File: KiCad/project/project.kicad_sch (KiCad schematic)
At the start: 27 parts, among them P1 TerminalBlock 5P 5.0mm, U1 DRV8313PWPR

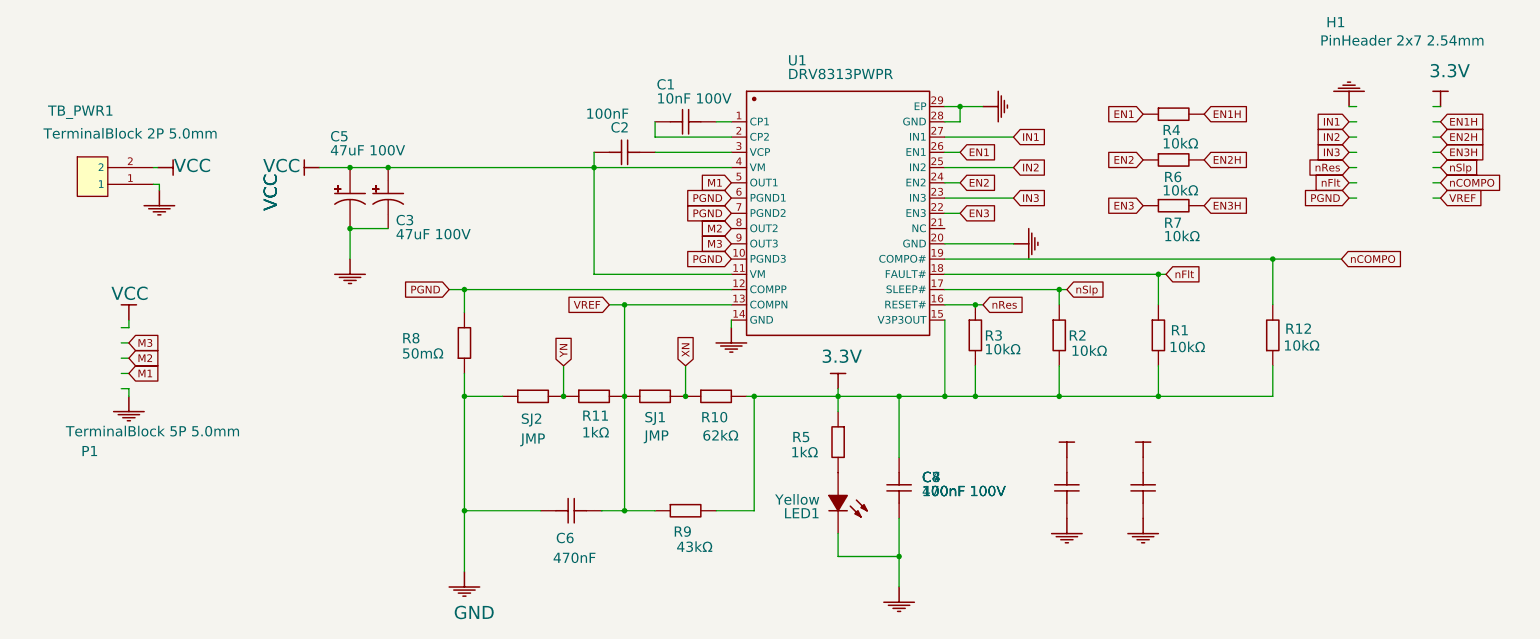
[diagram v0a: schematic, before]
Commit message: Claude's attempt at redoing the whole layout.
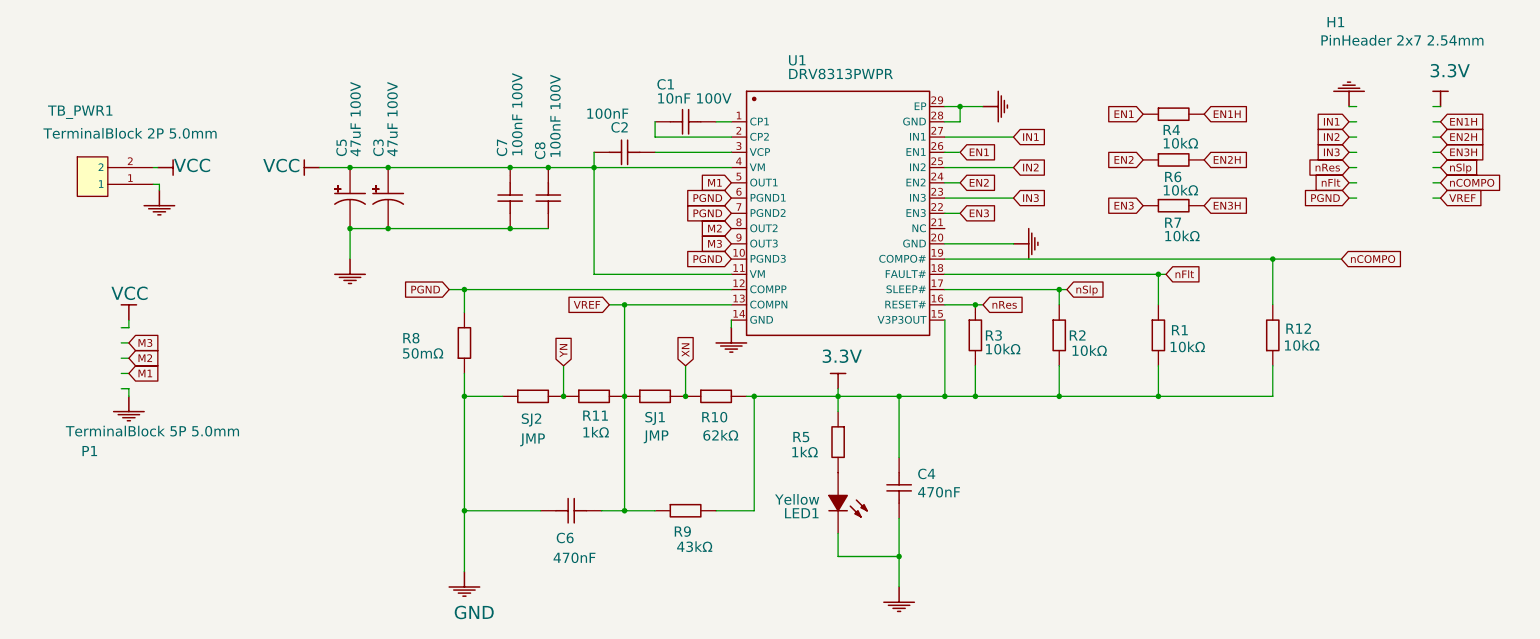
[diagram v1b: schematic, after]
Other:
- moved on the sheet: C7, C8
